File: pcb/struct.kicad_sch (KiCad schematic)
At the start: 28 parts

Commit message: Доработка структурной схемы
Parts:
- removed D?: ~, symbol struct:struct_arrow
- removed D?: ~, symbol struct:struct_oled
- added D1: ~, symbol struct:struct_sensors
- added D2, D3: ~, symbol struct:struct_arrow
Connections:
- net at DD?.: now also D?.
- new net: D2., D3.
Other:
- title: Система тестирования -> Автоматическая система управления

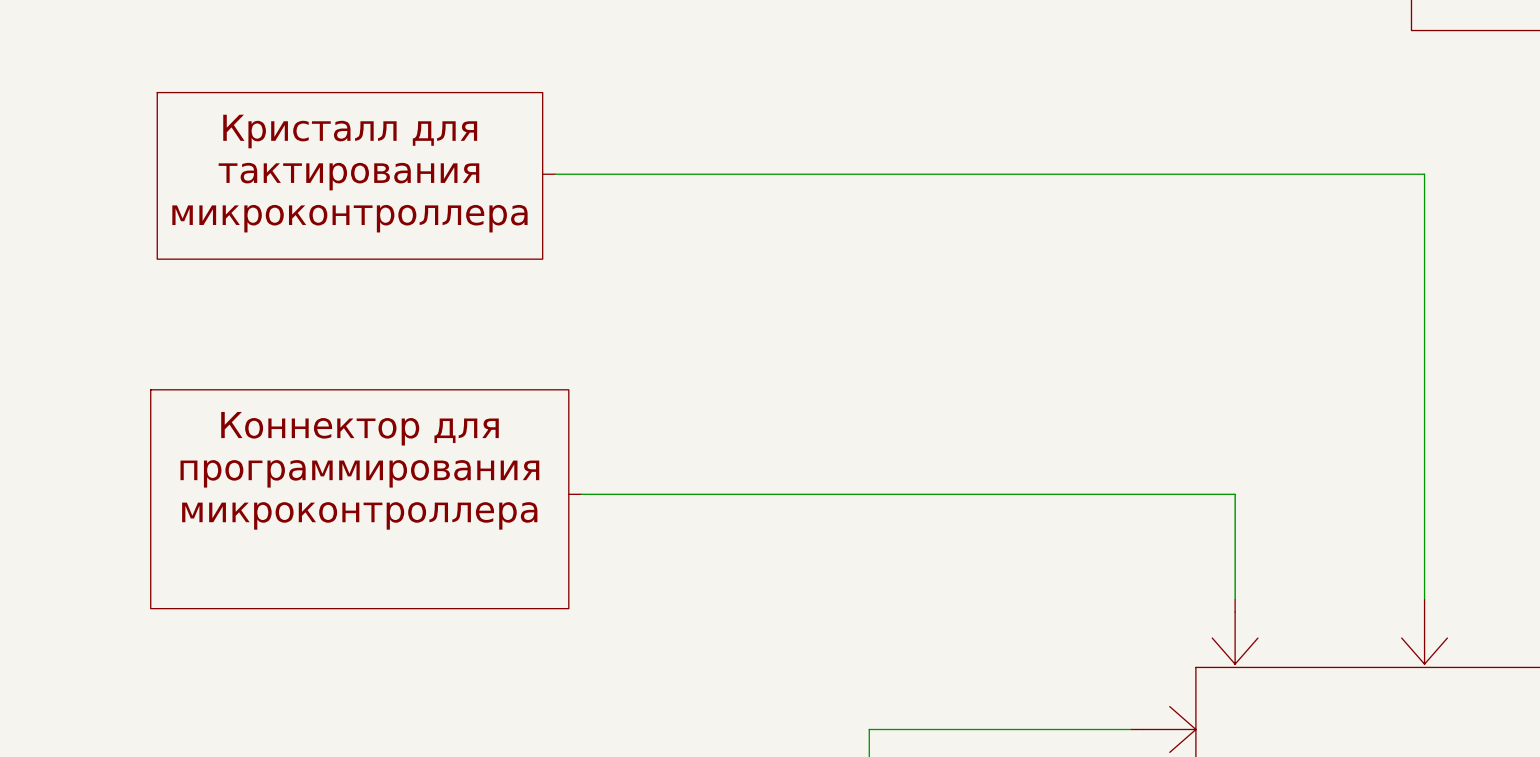
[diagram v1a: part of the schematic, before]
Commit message: Доработка структурной схемы
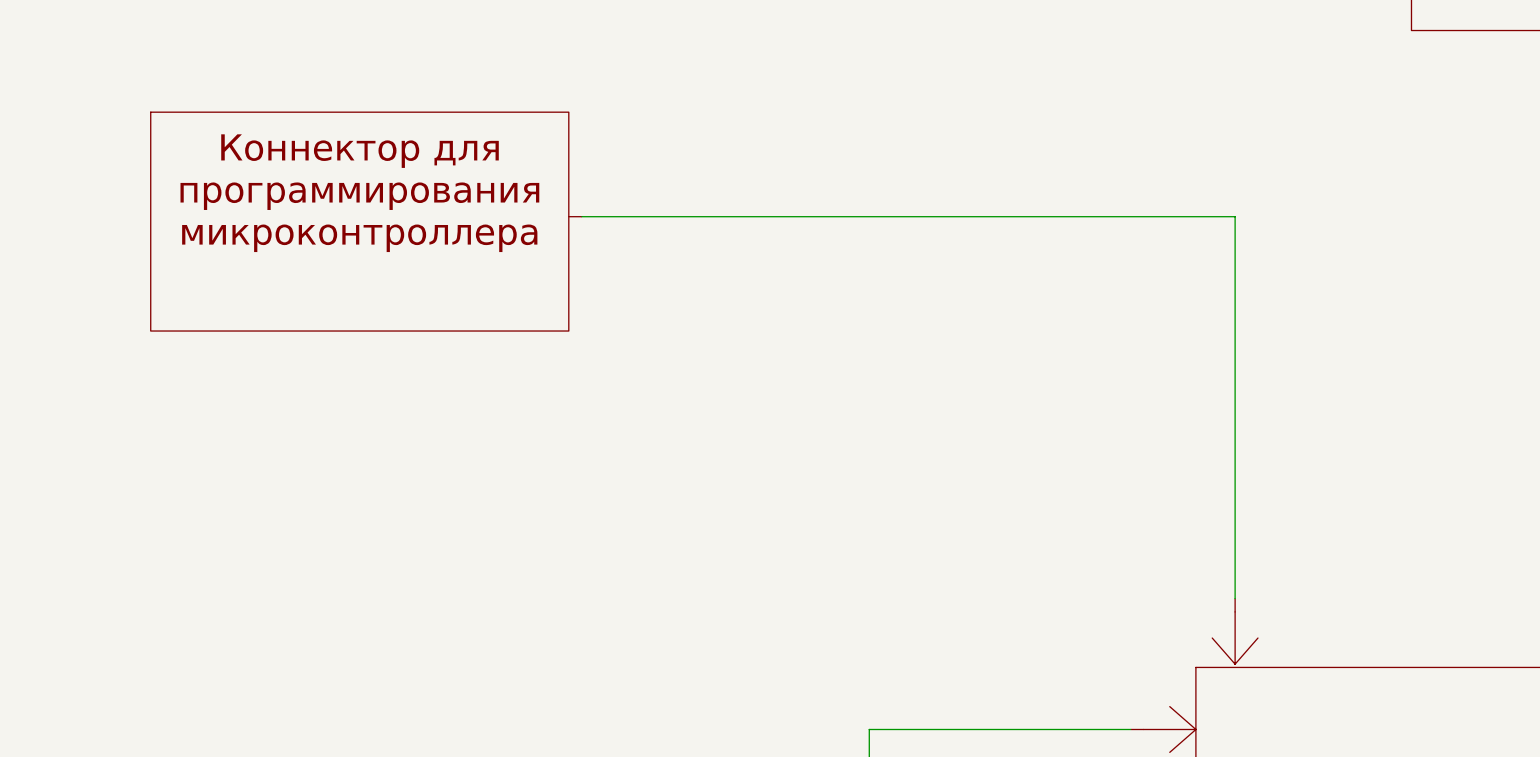
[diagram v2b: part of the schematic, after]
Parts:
- removed D?: ~, symbol struct:struct_arrow
- removed D?: ~, symbol struct:struct_ZQ
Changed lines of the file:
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@@
 	(title_block
 		(title "Автоматическая система управления")
-		(date "2025-03-23")
-		(comment 1 "46832.013 Э3")
+		(date "2025-05-02")
+		(comment 1 "467993.013 Э1")
 		(comment 2 "Корякин")
+		(comment 3 "Колбун")
+		(comment 4 "Алексеев")
+		(comment 6 "Ефремова")
 	)
 	(wire
@@
 	(wire
 		(pts
-			(xy 271.78 130.81) (xy 144.78 130.81)
+			(xy 271.78 76.835) (xy 144.78 76.835)
 		)
 		(stroke
@@
 	(wire
 		(pts
-			(xy 139.7 68.58) (xy 308.61 68.58)
-		)
-		(stroke
-			(width 0)
-			(type default)
-		)
-	)
-	(wire
-		(pts
 			(xy 180.975 377.19) (xy 307.34 377.19)
 		)
@@
 	(wire
 		(pts
-			(xy 308.61 68.58) (xy 308.61 151.13)
-		)
-		(stroke
-			(width 0)
-			(type default)
-		)
-	)
-	(wire
-		(pts
 			(xy 200.66 250.19) (xy 138.43 250.19)
 		)
@@
 	(wire
 		(pts
-			(xy 271.78 130.81) (xy 271.78 151.13)
+			(xy 271.78 76.835) (xy 271.78 151.13)
 		)
 		(stroke
@@
 	)
 	(symbol
-		(lib_id "struct:struct_arrow")
-		(at 308.61 151.13 270)
-		(unit 1)
-		(exclude_from_sim no)
-		(in_bom yes)
-		(on_board yes)
-		(dnp no)
-		(fields_autoplaced yes)
-		(property "Reference" "D?"
-			(at 313.69 158.1149 90)
-			(effects
-				(font
-					(size 1.27 1.27)
-				)
-				(justify left)
-				(hide yes)
-			)
-		)
-		(property "Value" "~"
-			(at 313.69 160.02 90)
-			(effects
-				(font
-					(size 1.27 1.27)
-				)
-				(justify left)
-			)
-		)
-		(property "Footprint" ""
-			(at 308.61 151.13 0)
-			(effects
-				(font
-					(size 1.27 1.27)
-				)
-				(hide yes)
-			)
-		)
-		(property "Datasheet" ""
-			(at 308.61 151.13 0)
-			(effects
-				(font
-					(size 1.27 1.27)
-				)
-				(hide yes)
-			)
-		)
-		(property "Description" ""
-			(at 308.61 151.13 0)
-			(effects
-				(font
-					(size 1.27 1.27)
-				)
-				(hide yes)
-			)
-		)
-		(pin ""
-		)
-		(instances
-			(project ""
-				(path "/ad8e3e9a-beb1-43ec-b57c-1a0280baf6c5"
-					(reference "D?")
-					(unit 1)
-				)
-			)
-		)
-	)
-	(symbol
 		(lib_id "struct:struct_supply_voltage")
 		(at 76.2 358.775 0)
@@
 	)
 	(symbol
-		(lib_id "struct:struct_ZQ")
-		(at 62.23 85.09 0)
-		(unit 1)
-		(exclude_from_sim no)
-		(in_bom yes)
-		(on_board yes)
-		(dnp no)
-		(fields_autoplaced yes)
-		(property "Reference" "D?"
-			(at 99.695 48.895 0)
-			(effects
-				(font
-					(size 1.27 1.27)
-				)
-				(hide yes)
-			)
-		)
-		(property "Value" "~"
-			(at 99.695 51.435 0)
-			(effects
-				(font
-					(size 1.27 1.27)
-				)
-			)
-		)
-		(property "Footprint" ""
-			(at 62.23 85.09 0)
-			(effects
-				(font
-					(size 1.27 1.27)
-				)
-				(hide yes)
-			)
-		)
-		(property "Datasheet" ""
-			(at 62.23 85.09 0)
-			(effects
-				(font
-					(size 1.27 1.27)
-				)
-				(hide yes)
-			)
-		)
-		(property "Description" ""
-			(at 62.23 85.09 0)
-			(effects
-				(font
-					(size 1.27 1.27)
-				)
-				(hide yes)
-			)
-		)
-		(pin ""
-		)
-		(instances
-			(project ""
-				(path "/ad8e3e9a-beb1-43ec-b57c-1a0280baf6c5"
-					(reference "D?")
-					(unit 1)
-				)
-			)
-		)
-	)
-	(symbol
 		(lib_id "struct:struct_conn_program")
-		(at 60.96 153.035 0)
-		(unit 1)
-		(exclude_from_sim no)
-		(in_bom yes)
-		(on_board yes)
-		(dnp no)
-		(fields_autoplaced yes)
-		(property "Reference" "D?"
-			(at 101.6 107.315 0)
-			(effects
-				(font
-					(size 1.27 1.27)
-				)
-				(hide yes)
-			)
-		)
-		(property "Value" "~"
-			(at 101.6 108.585 0)
-			(effects
-				(font
-					(size 1.27 1.27)
-				)
-			)
-		)
-		(property "Footprint" ""
-			(at 60.96 153.035 0)
-			(effects
-				(font
-					(size 1.27 1.27)
-				)
-				(hide yes)
-			)
-		)
-		(property "Datasheet" ""
-			(at 60.96 153.035 0)
-			(effects
-				(font
-					(size 1.27 1.27)
-				)
-				(hide yes)
-			)
-		)
-		(property "Description" ""
-			(at 60.96 153.035 0)
-			(effects
-				(font
+		(at 60.96 99.06 0)
+		(unit 1)
+		(exclude_from_sim no)
+		(in_bom yes)
+		(on_board yes)
+		(dnp no)
+		(fields_autoplaced yes)
+		(property "Reference" "D?"
+			(at 101.6 53.34 0)
+			(effects
+				(font
+					(size 1.27 1.27)
+				)
+				(hide yes)
+			)
+		)
+		(property "Value" "~"
+			(at 101.6 54.61 0)
+			(effects
+				(font
+					(size 1.27 1.27)
+				)
+			)
+		)
+		(property "Footprint" ""
+			(at 60.96 99.06 0)
+			(effects
+				(font
+					(size 1.27 1.27)
+				)
+				(hide yes)
+			)
+		)
+		(property "Datasheet" ""
+			(at 60.96 99.06 0)
+			(effects
+				(font
+					(size 1.27 1.27)
+				)
+				(hide yes)
+			)
+		)
+		(property "Description" ""
+			(at 60.96 99.06 0)
+			(effects
+				(font
